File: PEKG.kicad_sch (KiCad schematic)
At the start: 76 parts, among them J1 USB_C_Receptacle, J2 AudioJack3, U10 74LVC1G125, U11 74LVC1G125, U12 NCS21802DMR2G, U13 NCS21802DMR2G, U14 NCS21802DMR2G, U4 74LVC2G74, U5 TS5A63157DBV, U6 TS5A63157DBV, U7 TS5A63157DBV, U8 NCS21802DMR2G, U9 74LVC1G125

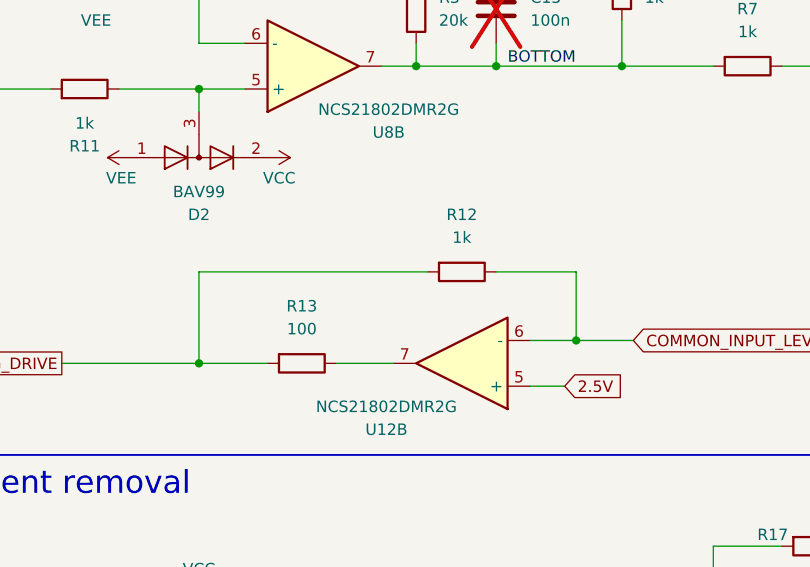
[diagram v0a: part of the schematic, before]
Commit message: Newwww
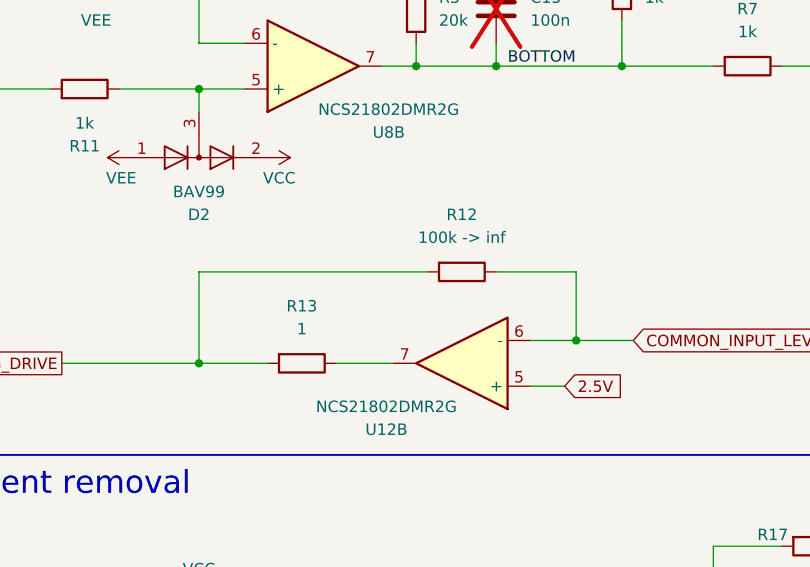
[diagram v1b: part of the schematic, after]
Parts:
- R12: value 1k -> 100k -> inf
- R13: value 100 -> 1
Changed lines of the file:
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@@
 			"AAAAAAAAAAAAAAAAAAAAAAAAAAAAAAAAAAAAAAAAAAAAAAAAAAAAAAAAAAAAAAAAAAAAAAAAAAAA"
 			"AAAAAAAAAAAAAAAAAAAAAAAAAAAAAAAAAAAAAAAAAAAAAAAAAAAAAAAAAAAAAAAAAAAAAAAAAAAA"
+			"AAAAAAAAAAAAAAAAAAAAAAAAAAAAAAAAAAAAAAAAAAAAAAAAAAAAAAAAAAAAAAAAAAAAAAAAAAAA"
+			"AAAAAAAAAAAAAAAAAAAAAAAAAAAAAAAAAAAAAAAAAAAAAAAAAAAAAAAAAAAAAAAAAAAAAAAAAAAA"
+			"AAAAAAAAAAAAAAAAAAAAAAAAAAAAAAAAAAAAAAAAAAAAAAAAAAAAAAAAAAAAAAAAAAAAAAAAAAAA"
+			"AAAAAAAAAAAAAAAAAAAAAAAAAAAAAAAAAAAAAAAAAAAAAAAAAAAAAAAAAAAAAAAAAAAAAAAAAAAA"
+			"AAAAAAAAAAAAAAAAAAAAAAAAAAAAAAAAAAAAAAAAAAAAAAAAAAAAAAAAAAAAAAAAAAAAAAAAAAAA"
+			"AAAAAAAAAAAAAAAAAAAAAAAAAAAAAAAAAAAAAAAAAAAAAAAAAAAAAAAAAAAAAAAAAAAAAAAAAAAA"
+			"AAAAAAAAAAAAAAAAAAAAAAAAAAAAAAAAAAAAAAAAAAAAAAAAAAAAAAAAAAAAAAAAAAAAAAAAAAAA"
+			"AAAAAAAAAAAAAAAAAAAAAAAAAAAAAAAAAAAAAAAAAAAAAAAAAAAAAAAAAAAAAAAAAAAAAAAAAAAA"
+			"AAAAAAAAAAAAAAAAAAAAAAAAAAAAAAAAAAAAAAAAAAAAAAAAAAAAAAAAAAAAAAAAAAAAAAAAAAAA"
+			"AAAAAAAAAAAAAAAAAAAAAAAAAAAAAAAAAAAAAAAAAAAAAAAAAAAAAAAAAAAAAAAAAAAAAAAAAAAA"
+			"AAAAAAAAAAAAAAAAAAAAAAAAAAAAAAAAAAAAAAAAAAAAAAAAAAAAAAAAAAAAAAAAAAAAAAAAAAAA"
+			"AAAAAAAAAAAAAAAAAAAAAAAAAAAAAAAAAAAAAAAAAAAAAAAAAAAAAAAAAAAAAAAAAAAAAAAAAAAA"
+			"AAAAAAAAAAAAAAAAAAAAAAAAAAAAAAAAAAAAAAAAAAAAAAAAAAAAAAAAAAAAAAAAAAAAAAAAAAAA"
+			"AAAAAAAAAAAAAAAAAAAAAAAAAAAAAAAAAAAAAAAAAAAAAAAAAAAAAAAAAAAAAAAAAAAAAAAAAAAA"
+			"AAAAAAAAAAAAAAAAAAAAAAAAAAAAAAAAAAAAAAAAAAAAAAAAAAAAAAAAAAAAAAAAAAAAAAAAAAAA"
+			"AAAAAAAAAAAAAAAAAAAAAAAAAAAAAAAAAAAAAAAAAAAAAAAAAAAAAAAAAAAAAAAAAAAAAAAAAAAA"
+			"AAAAAAAAAAAAAAAAAAAAAAAAAAAAAAAAAAAAAAAAAAAAAAAAAAAAAAAAAAAAAAAAAAAAAAAAAAAA"
+			"AAAAAAAAAAAAAAAAAAAAAAAAAAAAAAAAAAAAAAAAAAAAAAAAAAAAAAAAAAAAAAAAAAAAAAAAAAAA"
 			"AAAAAAAAAAAAAAAAAAAAAAAAAAAAAAAAAAAAAAAAAAAAAAAAAAAAAAAAAAAAAA=="
 		)
@@
 			)
 		)
-		(property "Value" "100"
+		(property "Value" "1"
 			(at 69.85 106.68 90)
 			(effects
@@
 			)
 		)
-		(property "Value" "1k"
+		(property "Value" "100k -> inf"
 			(at 87.63 96.52 90)
 			(effects
